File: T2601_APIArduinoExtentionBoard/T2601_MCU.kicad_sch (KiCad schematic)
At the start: 19 parts, among them J27 Conn_01x04, U2 ATmega328PB-A, X2 X322516MOB4SI

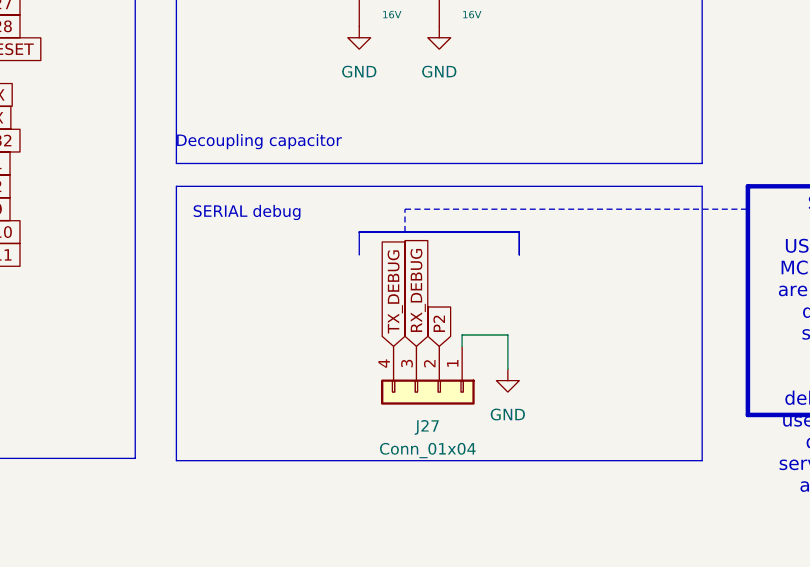
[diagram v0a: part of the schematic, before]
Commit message: Reroutage en cours 2
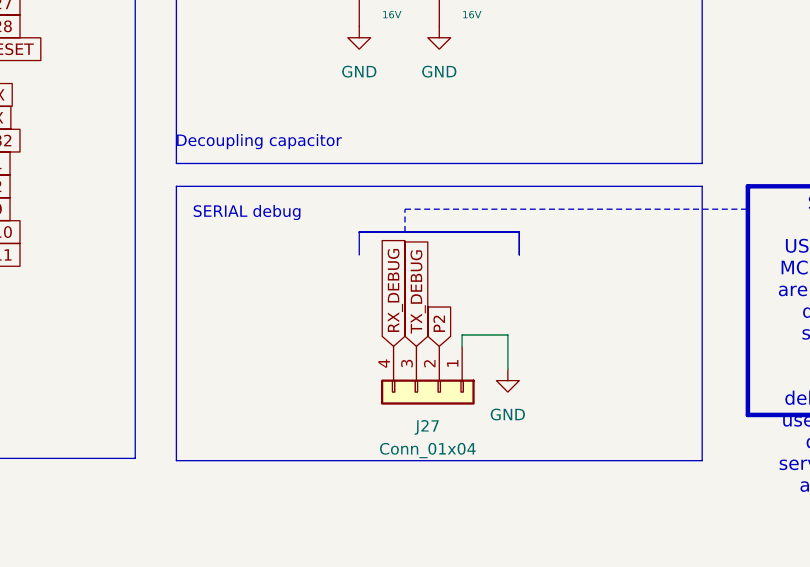
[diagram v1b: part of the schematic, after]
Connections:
- net RX_DEBUG: now also J27.4 (Pin_4); no longer J27.3 (Pin_3)
- net TX_DEBUG: now also J27.3 (Pin_3); no longer J27.4 (Pin_4)
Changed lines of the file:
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@@
 	(global_label "TX_DEBUG"
 		(shape input)
-		(at 209.55 127 90)
+		(at 212.09 127 90)
 		(fields_autoplaced yes)
 		(effects
@@
 		)
 		(property "Intersheetrefs" "${INTERSHEET_REFS}"
-			(at 209.55 114.5806 90)
+			(at 212.09 114.5806 90)
 			(hide yes)
 			(show_name no)
@@
 	(global_label "RX_DEBUG"
 		(shape input)
-		(at 212.09 127 90)
+		(at 209.55 127 90)
 		(fields_autoplaced yes)
 		(effects
@@
 		)
 		(property "Intersheetrefs" "${INTERSHEET_REFS}"
-			(at 212.09 114.2782 90)
+			(at 209.55 114.2782 90)
 			(hide yes)
 			(show_name no)
